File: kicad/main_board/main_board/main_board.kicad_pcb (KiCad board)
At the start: 2 copper layers, 2 parts, among them U1 AMS1117, U2 Pico

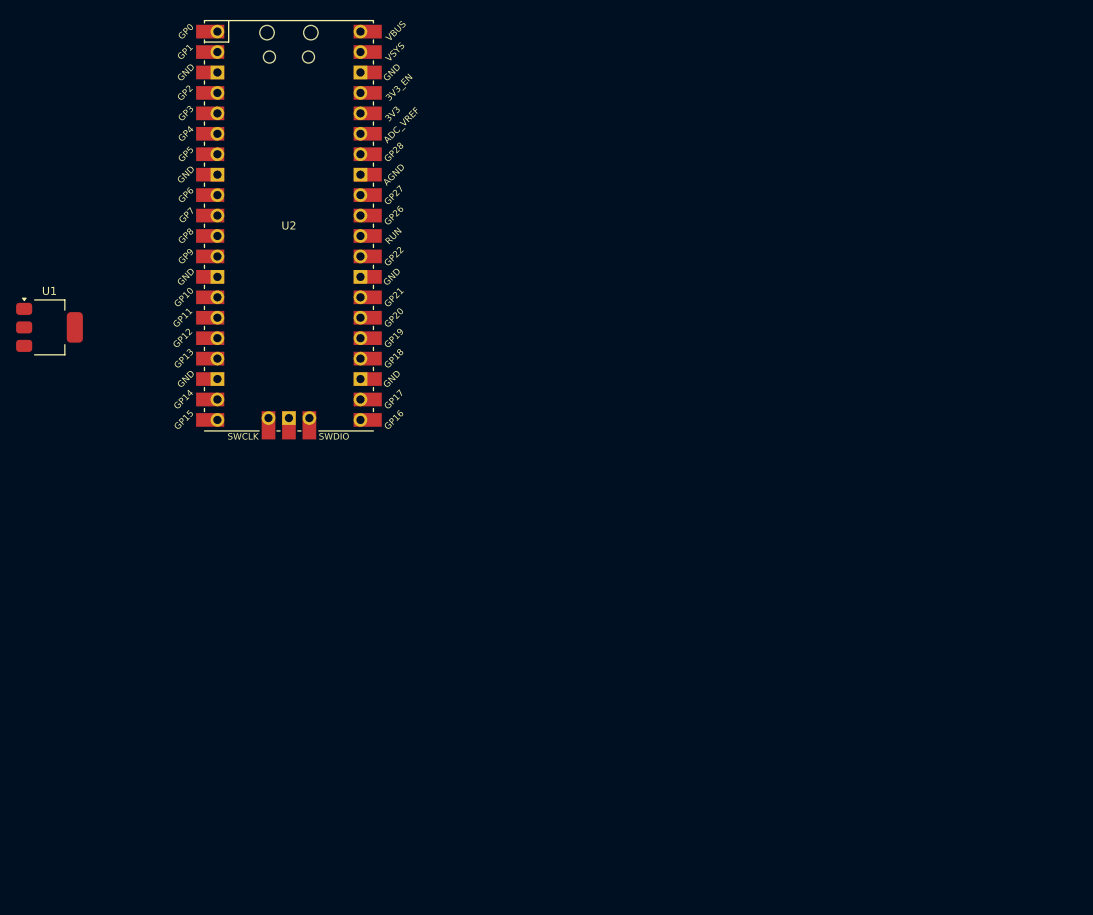
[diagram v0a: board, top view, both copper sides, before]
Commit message: [feat]final versions of boards + gerbers
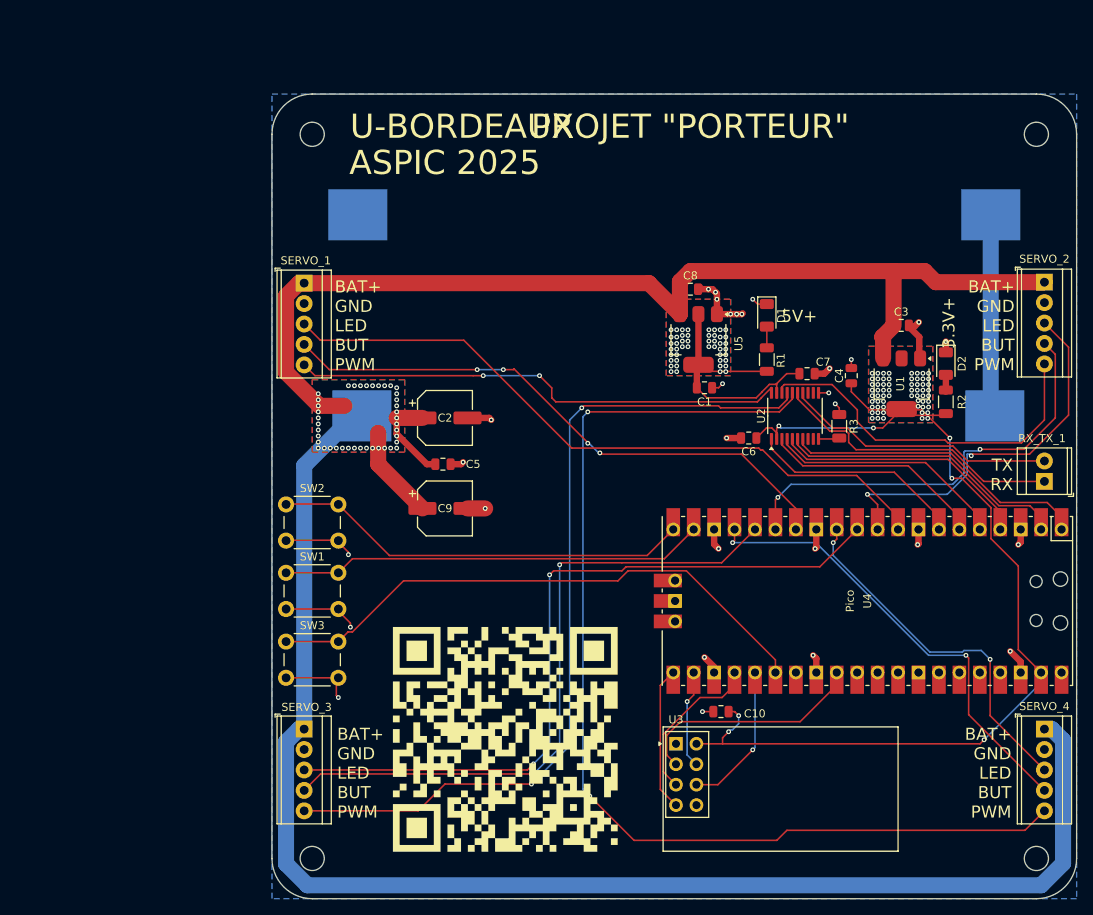
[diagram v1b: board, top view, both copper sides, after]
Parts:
- added BT1: Battery_Cell, Battery:BatteryHolder_Keystone_1042_1x18650, B.Cu at (150.5, 90.0)
- added BT2: Battery_Cell, Battery:BatteryHolder_Keystone_1042_1x18650, B.Cu at (150.0, 65.0)
- added C1: 1uf, Capacitor_SMD:C_0805_2012Metric, F.Cu at (153.8, 86.5)
- added C10: 1uf, Capacitor_SMD:C_0805_2012Metric, F.Cu at (155.8, 126.8)
- added C2: 10uf, Capacitor_SMD:CP_Elec_6.3x5.4, F.Cu at (121.5, 90.2)
- added C3: 1uf, Capacitor_SMD:C_0805_2012Metric, F.Cu at (178.2, 78.8)
- added C4: 1uf, Capacitor_SMD:C_0805_2012Metric, F.Cu at (172.0, 85.0)
- added C5: 1uf, Capacitor_SMD:C_0805_2012Metric, F.Cu at (121.2, 96.0)
- added C6: 1uf, Capacitor_SMD:C_0805_2012Metric, F.Cu at (159.2, 92.8)
- added C7: 1uf, Capacitor_SMD:C_0805_2012Metric, F.Cu at (166.5, 84.8)
- added C8: 1uf, Capacitor_SMD:C_0805_2012Metric, F.Cu at (152.0, 74.2)
- added C9: 10uf, Capacitor_SMD:CP_Elec_6.3x5.4, F.Cu at (121.5, 101.5)
- added D1: D, Diode_SMD:D_1206_3216Metric, F.Cu at (161.5, 77.5)
- added D2: D, Diode_SMD:D_1206_3216Metric, F.Cu at (183.8, 83.5)
- added G***: LOGO, LOGO, F.Cu at (129.0, 130.2)
- added H1: MountingHole, MountingHole:MountingHole_3mm, F.Cu at (105.0, 55.0)
- added H2: MountingHole, MountingHole:MountingHole_3mm, F.Cu at (195.0, 55.0)
- added H3: MountingHole, MountingHole:MountingHole_3mm, F.Cu at (105.0, 145.0)
- added H4: MountingHole, MountingHole:MountingHole_3mm, F.Cu at (195.0, 145.0)
- added R1: R, Resistor_SMD:R_1206_3216Metric, F.Cu at (161.5, 83.0)
- added R2: R, Resistor_SMD:R_1206_3216Metric, F.Cu at (183.8, 88.2)
- added R3: 10k, Resistor_SMD:R_1206_3216Metric, F.Cu at (170.5, 91.3)
- added RX_TX_1: Conn_01x02_Pin, TerminalBlock_TE-Connectivity:TerminalBlock_TE_282834-2_1x02_P2.54mm_Horizontal, F.Cu at (196.0, 98.1)
- added SERVO_1: Conn_01x05_Pin, TerminalBlock_TE-Connectivity:TerminalBlock_TE_282834-5_1x05_P2.54mm_Horizontal, F.Cu at (104.0, 73.5)
- added SERVO_2: Conn_01x05_Pin, TerminalBlock_TE-Connectivity:TerminalBlock_TE_282834-5_1x05_P2.54mm_Horizontal, F.Cu at (196.0, 73.4)
- added SERVO_3: Conn_01x05_Pin, TerminalBlock_TE-Connectivity:TerminalBlock_TE_282834-5_1x05_P2.54mm_Horizontal, F.Cu at (104.0, 128.9)
- added SERVO_4: Conn_01x05_Pin, TerminalBlock_TE-Connectivity:TerminalBlock_TE_282834-5_1x05_P2.54mm_Horizontal, F.Cu at (196.0, 128.9)
- added SW1: SW_Push, Button_Switch_THT:SW_PUSH_6mm, F.Cu at (101.8, 109.5)
- added SW2: SW_Push, Button_Switch_THT:SW_PUSH_6mm, F.Cu at (101.8, 101.0)
- added SW3: SW_Push, Button_Switch_THT:SW_PUSH_6mm, F.Cu at (101.8, 118.0)
- added U3: NRF24L01_Breakout, RF_Module:nRF24L01_Breakout, F.Cu at (150.2, 130.8)
- added U4: Pico, pi:RPi_Pico_SMD_TH, F.Cu at (174.0, 113.0)
- added U5: AMS1117, Package_TO_SOT_SMD:SOT-223-3_TabPin2, F.Cu at (153.0, 80.5)
- U2: value Pico -> TXS0108EPW; footprint MCU_RaspberryPi_and_Boards:RPi_Pico_SMD_TH -> Package_SO:TSSOP-20_4.4x6.5mm_P0.65mm
- moved U1 106.1 mm to (178.2, 86.0), turned to -90 degrees
- moved U2 67.2 mm to (165.0, 90.0), turned to 90 degrees
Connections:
- U2 pad 1: unconnected-(U2-GPIO0-Pad1) -> PWM_4_3v3
- U2 pad 10: unconnected-(U2-GPIO7-Pad10) -> Net-(U2-OE)
- U2 pad 11: unconnected-(U2-GPIO8-Pad11) -> GND
- U2 pad 14: unconnected-(U2-GPIO10-Pad14) -> TX
- U2 pad 15: unconnected-(U2-GPIO11-Pad15) -> RX
- U2 pad 16: unconnected-(U2-GPIO12-Pad16) -> PWM_4
- U2 pad 17: unconnected-(U2-GPIO13-Pad17) -> PWM_3
- U2 pad 18: unconnected-(U2-GND-Pad18) -> PWM_2
- U2 pad 19: unconnected-(U2-GPIO14-Pad19) -> 5V+
- U2 pad 2: unconnected-(U2-GPIO1-Pad2) -> 3.3V+
- U2 pad 20: unconnected-(U2-GPIO15-Pad20) -> PWM_1
- U2 pad 3: unconnected-(U2-GND-Pad3) -> PWM_3_3v3
- U2 pad 4: unconnected-(U2-GPIO2-Pad4) -> PWM_2_3v3
- U2 pad 5: unconnected-(U2-GPIO3-Pad5) -> PWM_1_3v3
- U2 pad 6: unconnected-(U2-GPIO4-Pad6) -> RX_3.3
- U2 pad 7: unconnected-(U2-GPIO5-Pad7) -> TX_3.3
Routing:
- net BAT+: track 0.00 -> 332.5 mm, vias 0 -> 41
- net PWM_4: track 0.00 -> 135.5 mm, vias 0 -> 2
- net 3.3V+: track 0.00 -> 132.3 mm, vias 0 -> 69
- net PWM_3: track 0.00 -> 106.0 mm, vias 0 -> 2
- net LED_3: track 0.00 -> 93.7 mm, vias 0 -> 2
- net LED_1: track 0.00 -> 85.3 mm
- net BUT_3: track 0.00 -> 82.8 mm, vias 0 -> 2
- net GND: track 0.00 -> 80.8 mm, vias 0 -> 29
- net BUT_1: track 0.00 -> 72.3 mm, vias 0 -> 4
- net TEST_3: track 0.00 -> 70.6 mm
- net PWM_1: track 0.00 -> 62.1 mm, vias 0 -> 2
- net BUT_4: track 0.00 -> 57.4 mm, vias 0 -> 2
- net BUT_2: track 0.00 -> 54.0 mm, vias 0 -> 2
- net TEST_1: track 0.00 -> 52.9 mm
- net TEST_2: track 0.00 -> 52.1 mm
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- added copper zone on B.Cu, net 3.3V+
- added copper zone on F.Cu, net 3.3V+
- added copper zone on B.Cu, net 5V+
- added copper zone on F.Cu, net 5V+
- added copper zone on B.Cu, net BAT+
- added copper zone on F.Cu, net BAT+
- added copper zone on B.Cu, net GND
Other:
- board outline added: 100 x 100 mm
- board text added: "3.3V+"
- board text added: "5V+"
- board text added: "ASPIC 2025"
- board text added: "BAT+ GND LED BUT PWM"
- board text added: "C4"
- board text added: "DESIGNED by Gaetan {dblquote}TWIM{dblquote} CANTELOBRE"
- board text added: "PROJET {dblquote}PORTEUR{dblquote}"
- board text added: "TX RX"
- board text added: "U-BORDEAUX"
